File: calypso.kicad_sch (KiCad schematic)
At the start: 3 parts, among them J1 Conn_02x05_Odd_Even, J2 Conn_02x12_Odd_Even, J5 Conn_01x03

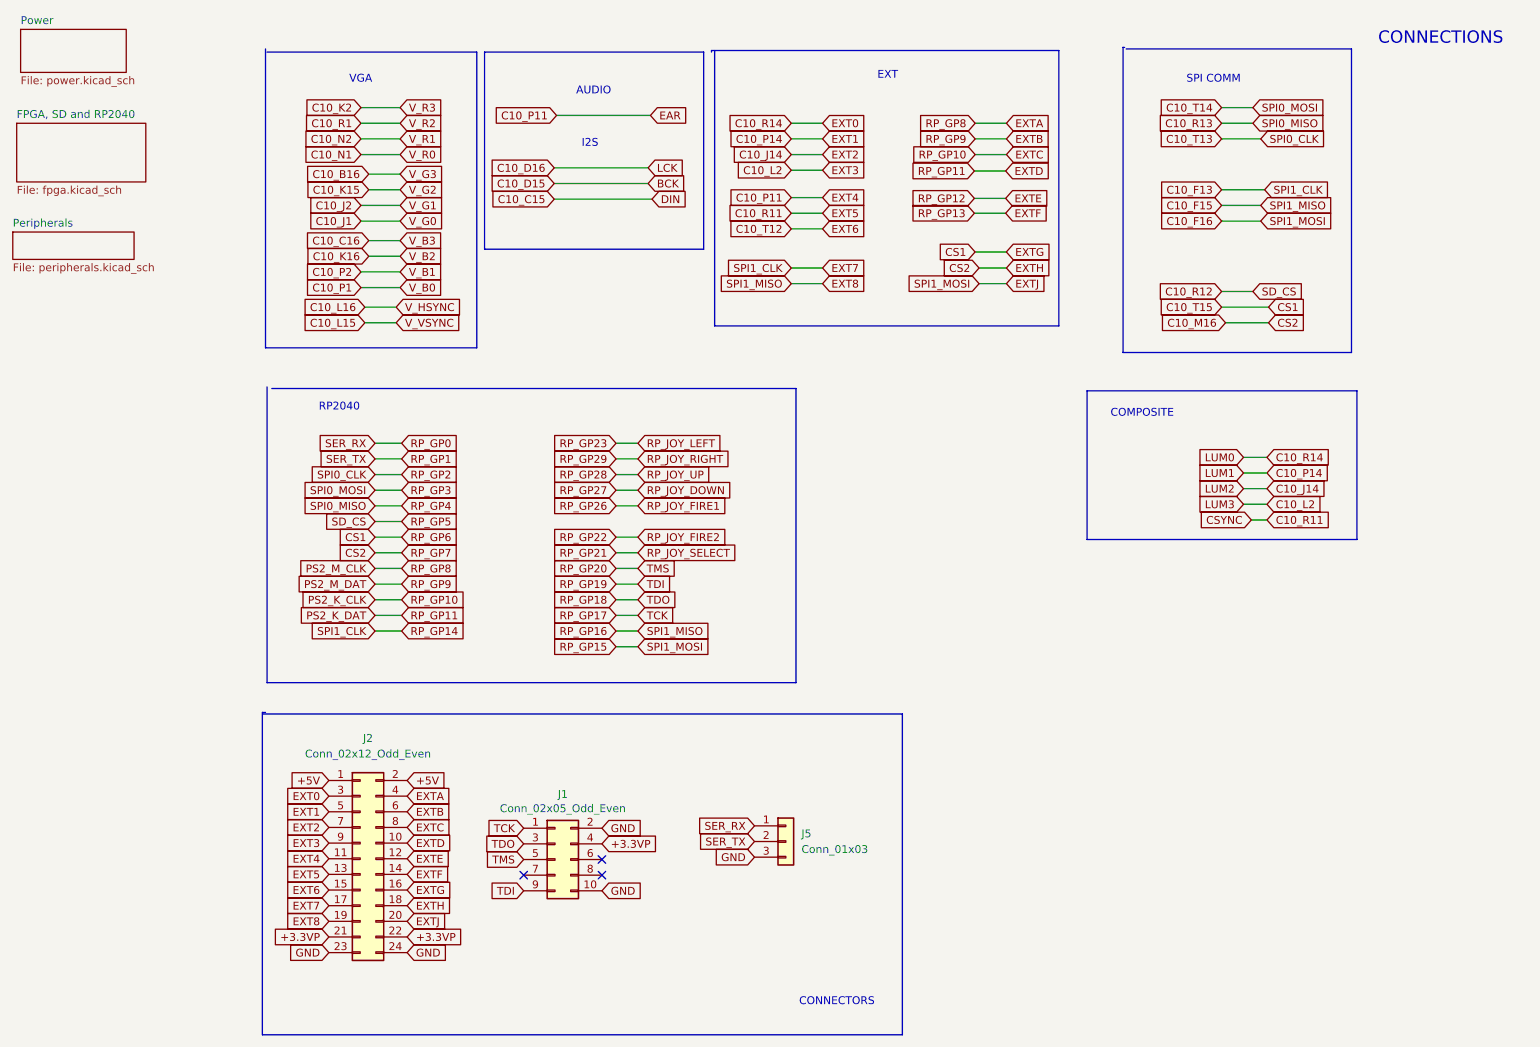
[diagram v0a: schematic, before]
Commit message: Version 0.2
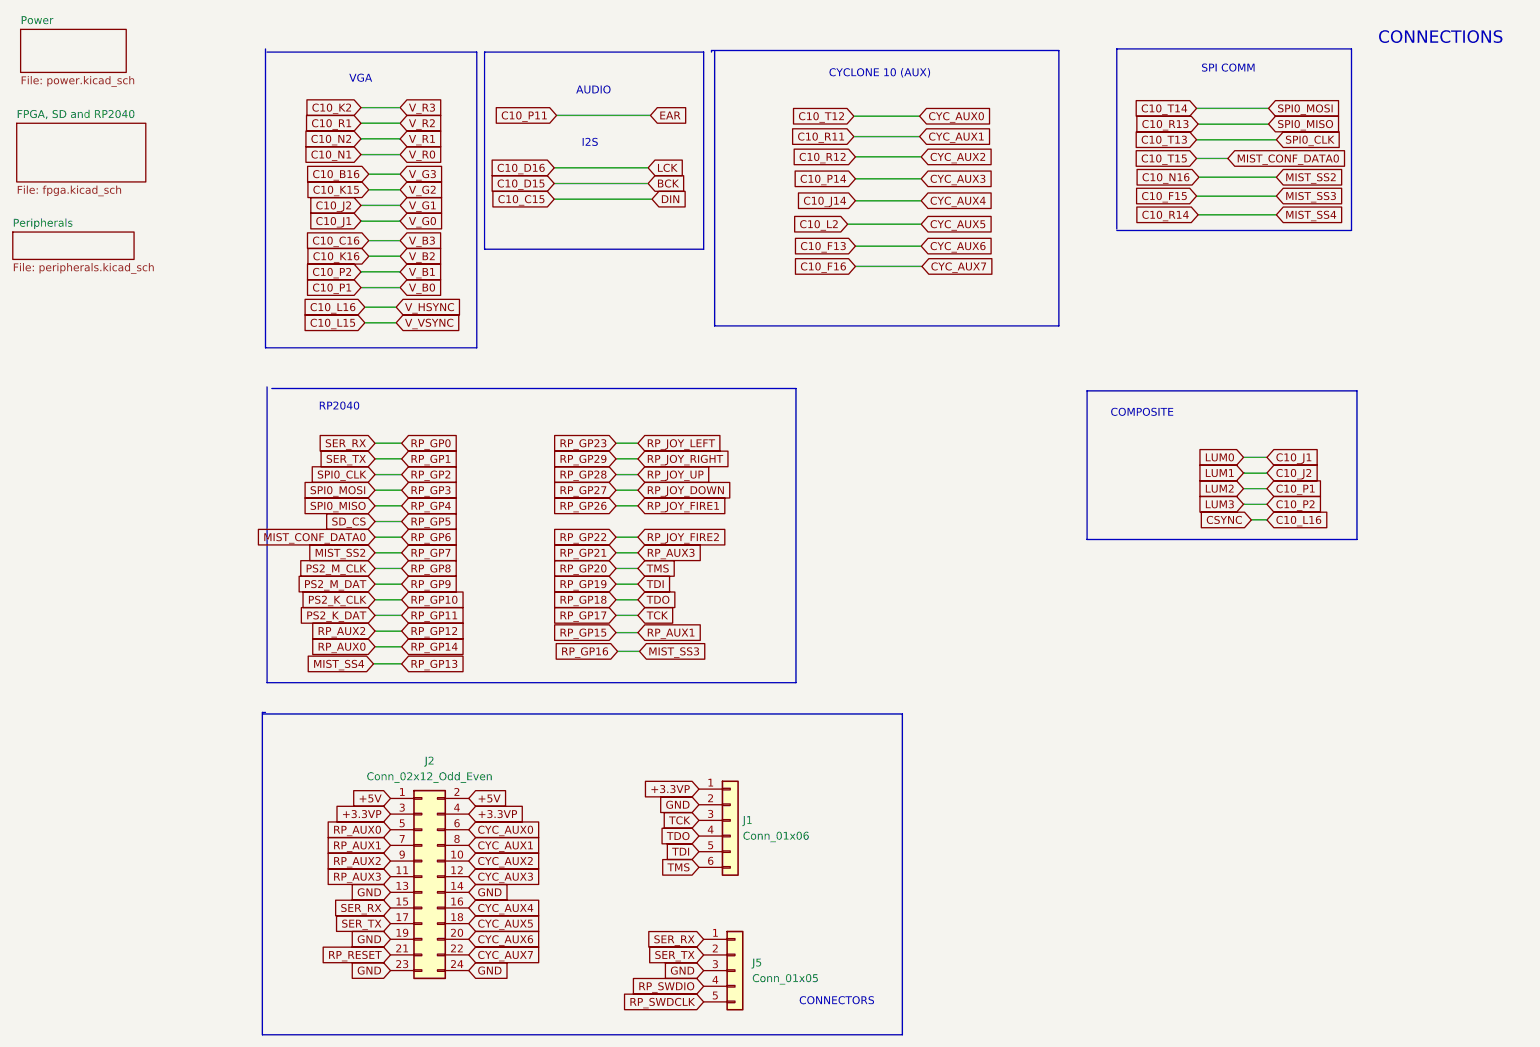
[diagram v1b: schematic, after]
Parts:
- removed J1: Conn_02x05_Odd_Even, Connector_PinHeader_2.54mm:PinHeader_2x05_P2.54mm_Vertical, symbol Connector_Generic:Conn_02x05_Odd_Even
- removed J5: Conn_01x03, Connector_PinHeader_2.54mm:PinHeader_1x03_P2.54mm_Vertical, symbol Connector_Generic:Conn_01x03
- added J1: Conn_01x06, Connector_PinHeader_2.54mm:PinHeader_1x06_P2.54mm_Vertical, symbol Connector_Generic:Conn_01x06
- added J5: Conn_01x05, Connector_PinHeader_2.54mm:PinHeader_1x05_P2.54mm_Vertical, symbol Connector_Generic:Conn_01x05
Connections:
- net C10_M16 is gone; now on net C10_L2: J2.18 (Pin_18)
- net EXTA is gone; now on net +3.3VP: J2.4 (Pin_4)
- net EXTB is gone; now on net C10_T12: J2.6 (Pin_6)
- net EXTC is gone; now on net C10_R11: J2.8 (Pin_8)
- net EXTD is gone; now on net C10_R12: J2.10 (Pin_10)
- net EXTE is gone; now on net C10_P14: J2.12 (Pin_12)
- net EXTF is gone; now on net GND: J2.14 (Pin_14)
- net +3.3VP: now also J2.3 (Pin_3), J1.1 (Pin_1); no longer J2.21 (Pin_21), J2.22 (Pin_22)
- net C10_F13: now also J2.20 (Pin_20); no longer J2.17 (Pin_17)
- net C10_F15: no longer J2.19 (Pin_19)
- net C10_F16: now also J2.22 (Pin_22); no longer J2.20 (Pin_20)
- net C10_J14: now also J2.16 (Pin_16); no longer J2.7 (Pin_7)
- net C10_L2: no longer J2.9 (Pin_9)
- net C10_P11: no longer J2.11 (Pin_11)
- net C10_P14: no longer J2.5 (Pin_5)
- net C10_R11: no longer J2.13 (Pin_13)
- net C10_R14: no longer J2.3 (Pin_3)
- net C10_T12: no longer J2.15 (Pin_15)
- net C10_T15: no longer J2.16 (Pin_16)
- net GND: now also J2.13 (Pin_13), J2.19 (Pin_19), J1.2 (Pin_2), J5.3 (Pin_3)
- net RP_GP0: now also J2.15 (Pin_15), J5.1 (Pin_1)
- net RP_GP1: now also J2.17 (Pin_17), J5.2 (Pin_2)
- net RP_GP17: now also J1.3 (Pin_3)
- net RP_GP18: now also J1.4 (Pin_4)
- net RP_GP19: now also J1.5 (Pin_5)
- net RP_GP20: now also J1.6 (Pin_6)
- new net RP_AUX0: J2.5 (Pin_5)
- new net RP_AUX1: J2.7 (Pin_7)
- new net RP_AUX2: J2.9 (Pin_9)
- new net RP_AUX3: J2.11 (Pin_11)
- new net RP_RESET: J2.21 (Pin_21)
- new net RP_SWDCLK: J5.5 (Pin_5)
- new net RP_SWDIO: J5.4 (Pin_4)
- no-connect marks 3 -> 0
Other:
- note added: "CYCLONE 10 (AUX)"
- note removed: "EXT"
- title: Calypso - was Atlas -> Calypso
